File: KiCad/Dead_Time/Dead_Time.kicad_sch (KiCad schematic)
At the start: 13 parts, among them Q7 PNP_BC558, U1 74AUC2G04, U2 MCP6002

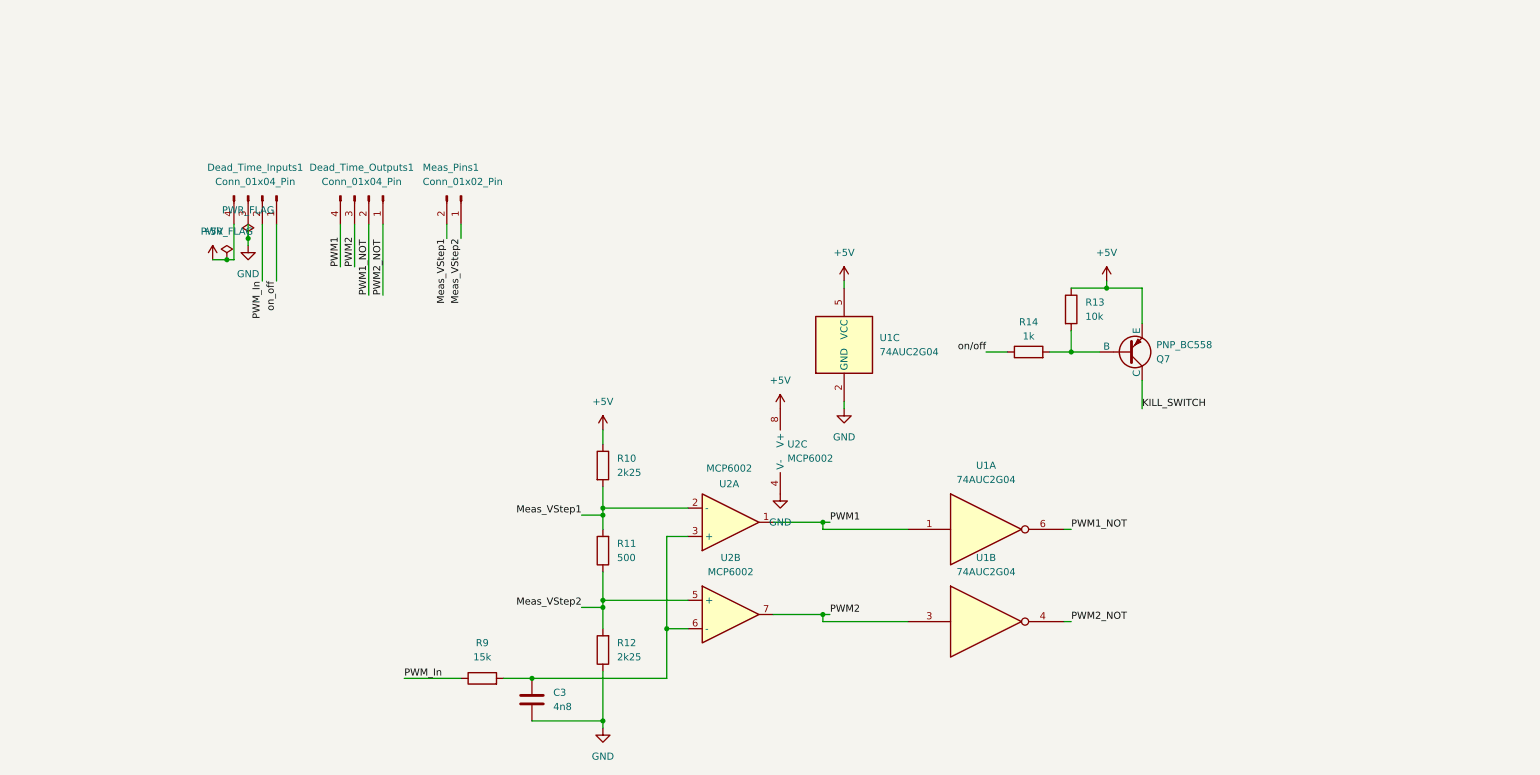
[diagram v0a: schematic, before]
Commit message: gemme punkt før jeg laver om i deadtime pcb
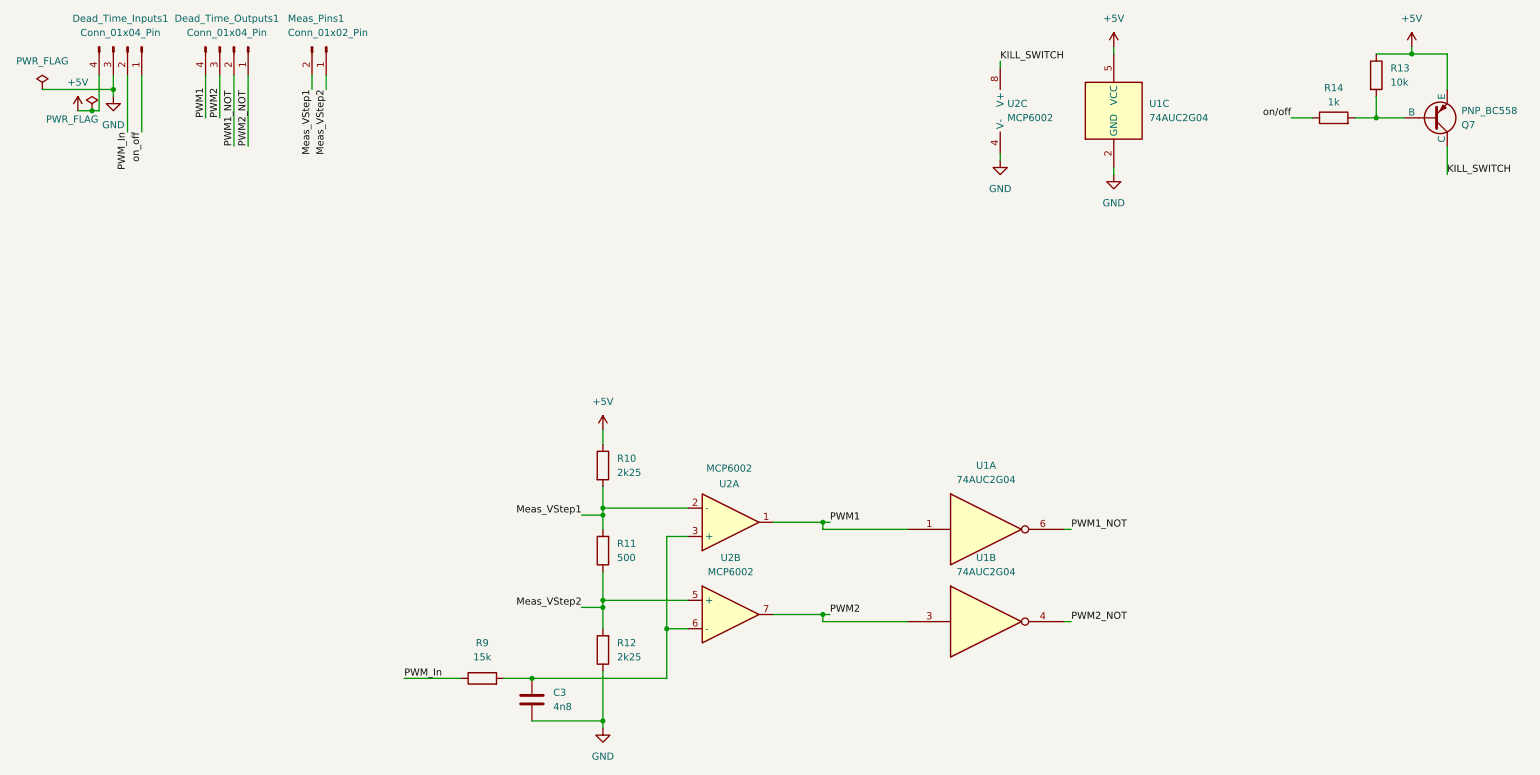
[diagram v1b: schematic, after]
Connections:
- net +5V: no longer U2.8 (V+)
- net KILL_SWITCH: now also U2.8 (V+)
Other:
- moved on the sheet: Dead_Time_Inputs1, Dead_Time_Outputs1, Meas_Pins1, Q7, R13, R14, U1C, U2C
